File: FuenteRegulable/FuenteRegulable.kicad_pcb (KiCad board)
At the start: 2 copper layers, 56 parts, among them J1 AC_IN, J2 OUT-P, J3 OUT-N, J4 OLED_I2C, Q1 IRF540N, Q2 2N3904, Q3 2N7000, Q4 IRF540N, Q5 2N3904, SW1 SW_MEC_5E, SW2 SW_MEC_5E, SW3 SW_MEC_5E, SW4 SW_MEC_5E, SW5 SW_MEC_5E, SW6 SW_MEC_5E, U2 LM2576T-5, U3 AMS1117-3.3, U4 TL082

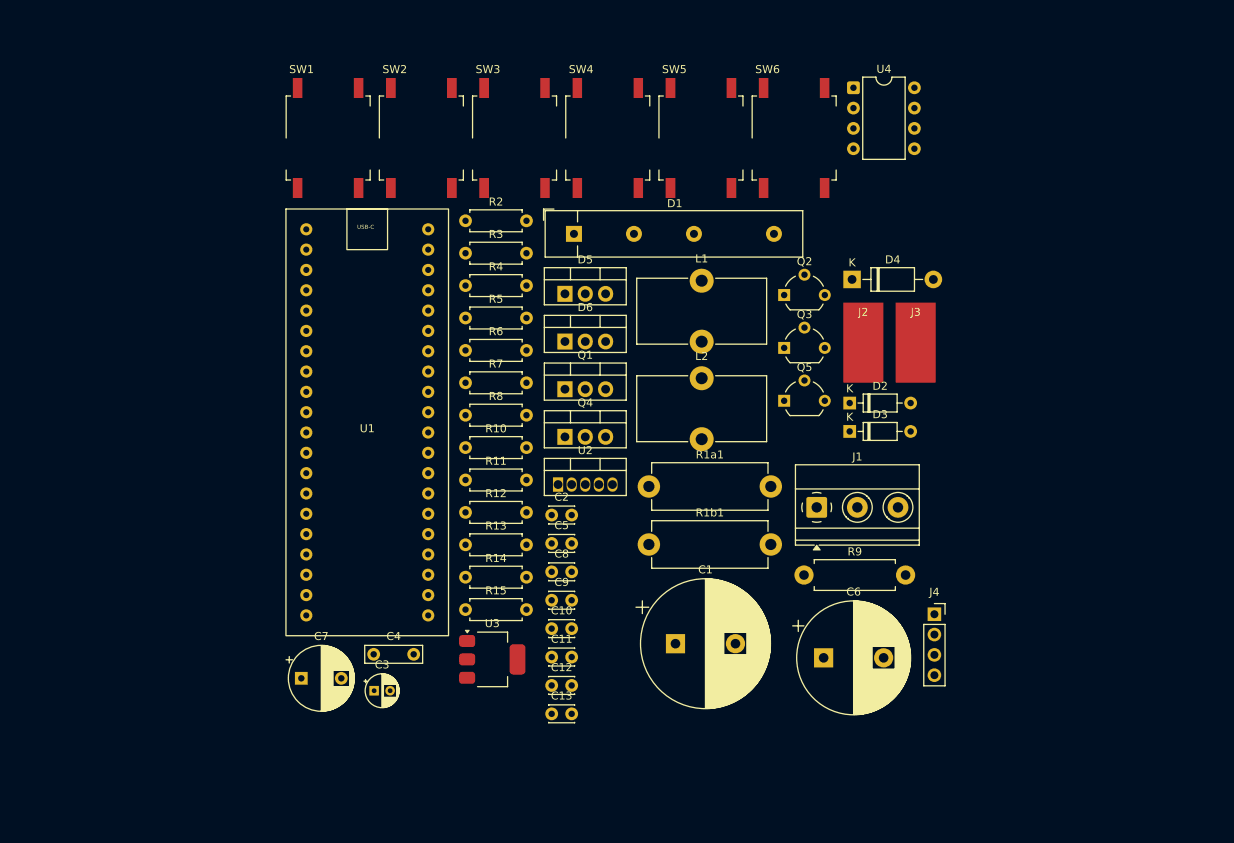
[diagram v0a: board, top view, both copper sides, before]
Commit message: Comienzo a rutear PCB
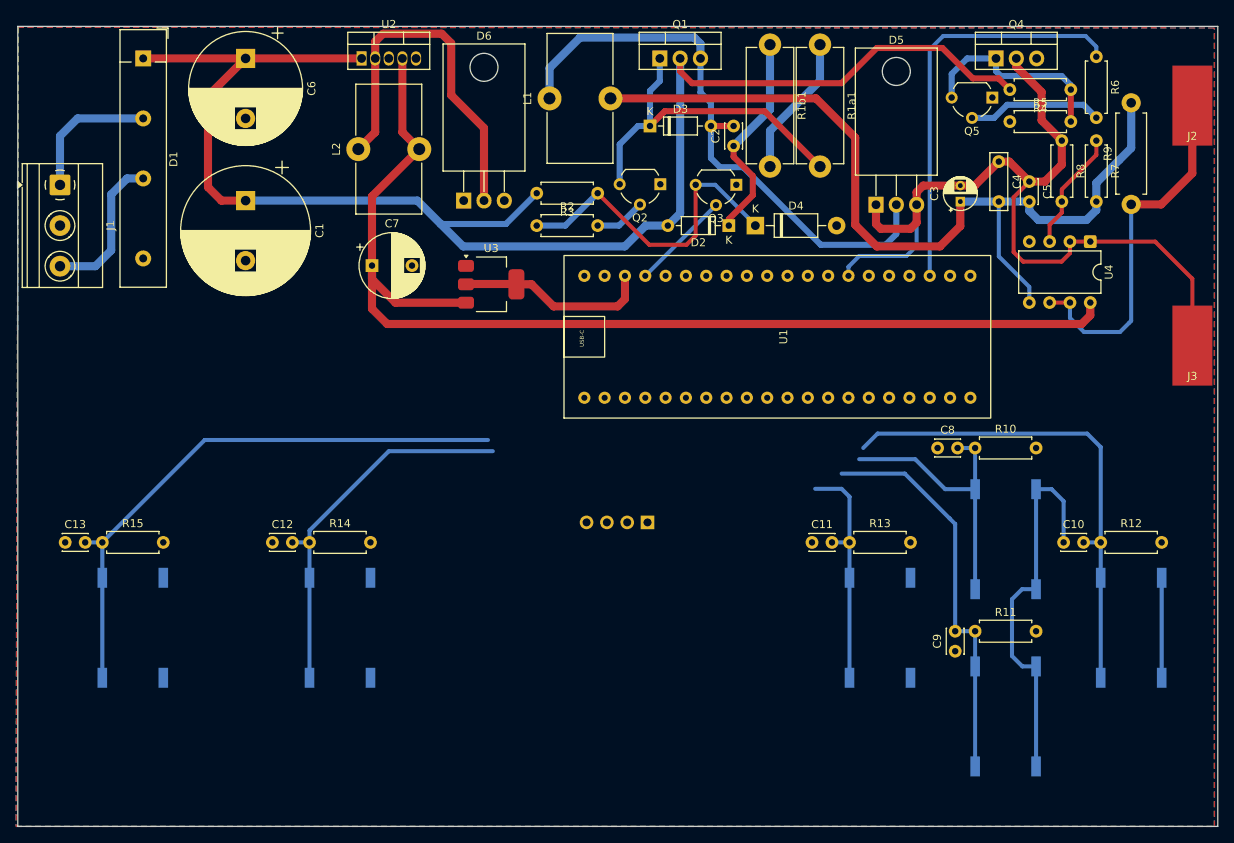
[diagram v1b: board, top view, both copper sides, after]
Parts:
- D5, D6: footprint Package_TO_SOT_THT:TO-220-3_Vertical -> Package_TO_SOT_THT:TO-220-3_Horizontal_TabDown
- J4, SW1, SW2, SW3, SW4, SW5, SW6: moved to B.Cu
- moved C6 104.1 mm to (99.4, 50.9), turned to -90 degrees
- moved SW6 102.9 mm to (85.3, 122.1), turned to 180 degrees
- moved J1 102.8 mm to (76.2, 66.7), turned to -90 degrees
- moved SW2 102.8 mm to (194.4, 133.2), turned to 180 degrees
- moved C4 99.5 mm to (193.6, 63.8), turned to -90 degrees
- moved SW3 98.4 mm to (210.1, 122.1), turned to 180 degrees
- moved SW1 98.4 mm to (194.4, 111.0), turned to 180 degrees
- moved C3 95.4 mm to (188.7, 68.8), turned to 90 degrees
- moved R6 87.0 mm to (205.7, 50.7), turned to -90 degrees
- moved R7 84.5 mm to (205.7, 61.2), turned to -90 degrees
- moved R8 82.1 mm to (201.4, 61.2), turned to -90 degrees
- moved R4 79.5 mm to (202.6, 54.8), turned to 180 degrees
- moved R12 79.5 mm to (206.3, 111.4)
- moved C1 77.2 mm to (99.4, 68.7), turned to -90 degrees
- moved SW5 76.1 mm to (111.2, 122.1), turned to 180 degrees
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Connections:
- J4 pad 1: +3V3 -> GND
- J4 pad 2: GND -> +3V3
- J4 pad 3: I2C_SDA -> I2C_SCL
- J4 pad 4: I2C_SCL -> I2C_SDA
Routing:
- net /Vs: track 0.00 -> 189.5 mm
- net +5V: track 0.00 -> 141.9 mm
- net Io_MeasP: track 0.00 -> 110.5 mm
- net Load_N: track 0.00 -> 109.6 mm
- net Net-(D3-A): track 0.00 -> 74.1 mm
- net BTN_RETURN: track 0.00 -> 72.6 mm
- net BTN_PLUS: track 0.00 -> 62.1 mm
- net GND: track 0.00 -> 60.9 mm
- net SHUTDOWN: track 0.00 -> 51.6 mm
- net BTN_DOWN: track 0.00 -> 49.6 mm
- net BTN_ENTER: track 0.00 -> 47.6 mm
- net Net-(D6-K): track 0.00 -> 46.1 mm
- net Io_ADC: track 0.00 -> 45.7 mm
- net Net-(D3-K): track 0.00 -> 43.6 mm
- net Net-(D4-K): track 0.00 -> 40.7 mm
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- added copper zone on B.Cu, net GND
- added copper zone on F.Cu, net GND
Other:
- board outline added: 150 x 100 mm
